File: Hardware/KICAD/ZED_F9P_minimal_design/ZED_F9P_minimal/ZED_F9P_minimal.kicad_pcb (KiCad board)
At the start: 2 copper layers, 71.5 x 55.5 mm, 28 parts, among them J1 Conn_Coaxial_Small, J2 DF11-18DS-2DSA06, U1 OPA2365AID, U2 LM1086IT-ADJ/NOPB, U3 ZED-F9P

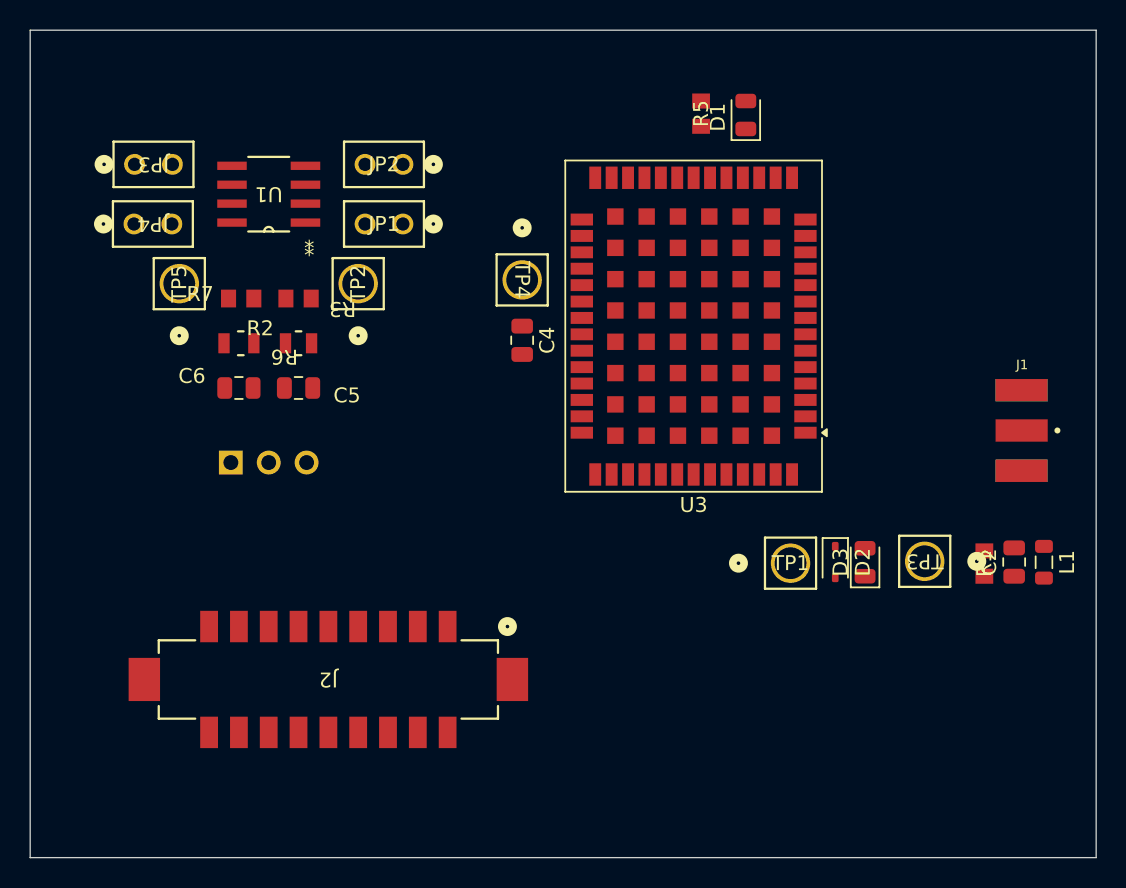
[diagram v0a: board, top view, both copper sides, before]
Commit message: rooting pcb
work in progerss
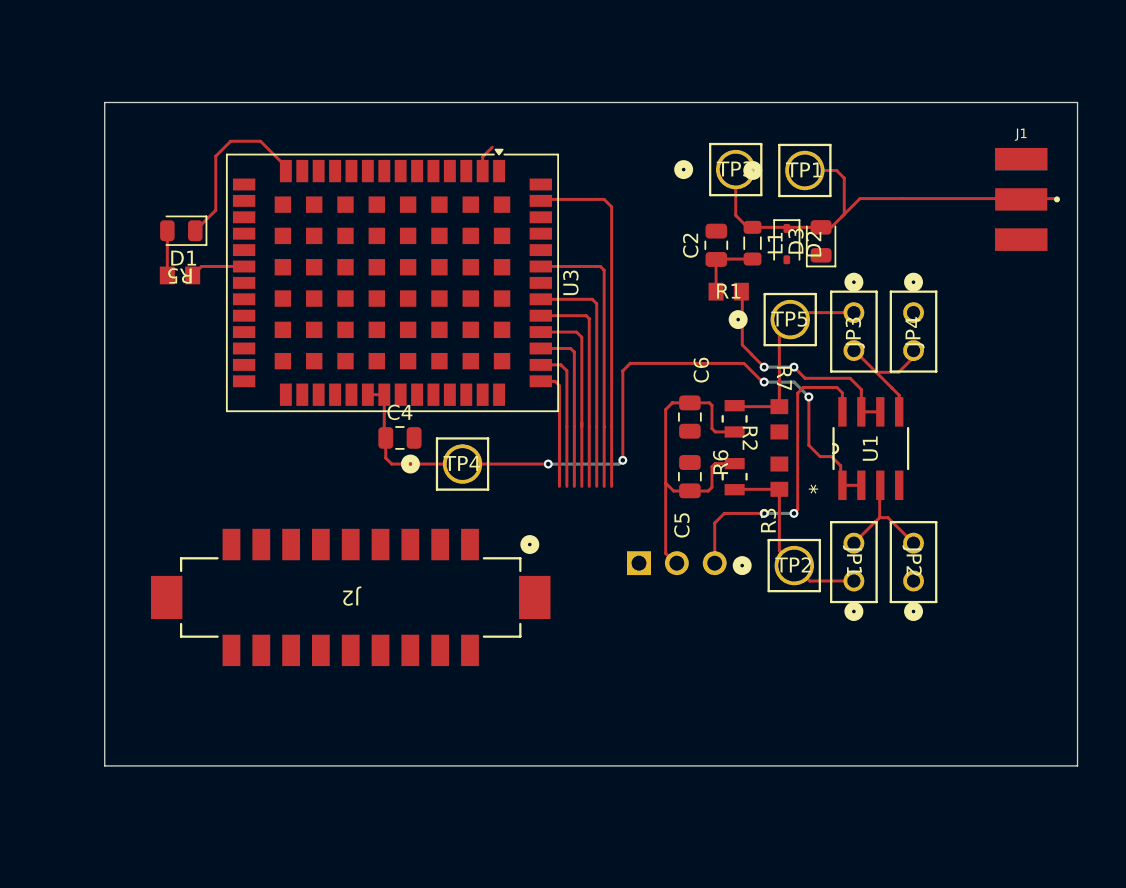
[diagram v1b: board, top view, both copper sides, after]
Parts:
- moved JP4 52.6 mm to (71.2, 30.9), turned to 90 degrees
- moved JP3 49.3 mm to (67.2, 30.9), turned to 90 degrees
- moved JP2 44.2 mm to (71.2, 48.9), turned to -90 degrees
- moved U1 43.8 mm to (68.4, 40.1), turned to 90 degrees
- moved TP5 41.1 mm to (63.0, 31.4), turned to 0 degrees
- moved D1 38.7 mm to (22.1, 25.4), turned to 180 degrees
- moved JP1 38.6 mm to (67.2, 48.9), turned to -90 degrees
- moved R7 37.0 mm to (62.2, 38.1), turned to -90 degrees
- moved R5 36.6 mm to (22.0, 28.4), turned to 180 degrees
- moved TP2 34.8 mm to (63.2, 47.9), turned to 0 degrees
- moved R3 34.4 mm to (62.2, 41.9), turned to 90 degrees
- moved R6 33.5 mm to (59.2, 38.1), turned to 90 degrees
- moved R2 30.6 mm to (59.2, 41.9), turned to -90 degrees
- moved C6 30.3 mm to (56.2, 37.9), turned to -90 degrees
- moved TP3 29.2 mm to (59.3, 21.4), turned to 0 degrees
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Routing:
- net /3v3_puce: track 0.00 -> 49.8 mm, vias 0 -> 4
- net /RF_IN: track 0.00 -> 33.3 mm
- net Net-(U2-OUTPUT): track 0.00 -> 24.2 mm
- net /TIMER: track 0.00 -> 23.7 mm
- net /12V: track 0.00 -> 21.0 mm, vias 0 -> 2
- net /I_RESET: track 0.00 -> 18.9 mm
- net /I_D_Sel: track 0.00 -> 16.1 mm
- net /5v_antenne: track 0.00 -> 16.0 mm, vias 0 -> 2
- net /O_TX_STATE: track 0.00 -> 14.6 mm
- net /5V-IN: track 0.00 -> 13.6 mm
- net /I/O_CLK_SELECT: track 0.00 -> 13.1 mm
- net /3V3-IN: track 0.00 -> 13.0 mm
- net GND: track 0.00 -> 12.0 mm
- net /I/O : track 0.00 -> 11.4 mm
- net /UART_RX: track 0.00 -> 9.67 mm
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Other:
- board size 71.5 x 55.5 mm -> 65.2 x 44.5 mm
